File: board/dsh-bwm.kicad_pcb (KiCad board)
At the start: 2 copper layers, 137.4 x 88.5 mm, 67 parts, among them IC1 MAX485CSA+T, IC2 AT24C256C-SSHL-T, IC3 TPS5450DDA, J1 USB_A, J2 MPM-15-24, J3 Power, J4 LED, J5 SWD6p, J6 Connections, K1 T81N5D312, K2 T81N5D312, K3 T81N5D312, K4 T81N5D312, K5 T81N5D312, K6 T81N5D312, K7 T81N5D312, K8 T81N5D312, Q1 IRLB8721PBF, Q2 IRLB8721PBF, Q3 IRLB8721PBF, Q4 IRLB8721PBF, Q5 IRLB8721PBF, Q6 IRLB8721PBF, SW1 ModBus address selector, SW2 RESET, U1 RP2040_Stamp

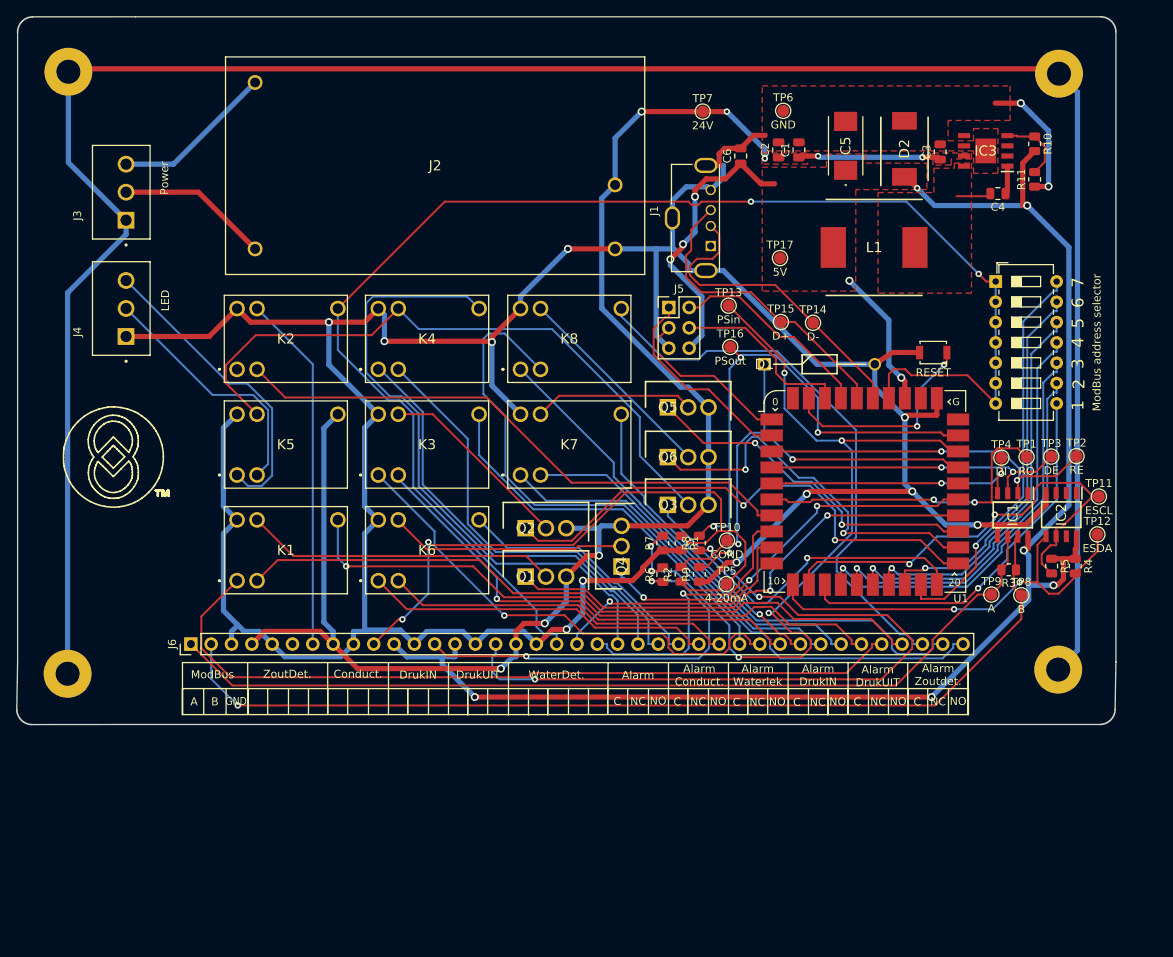
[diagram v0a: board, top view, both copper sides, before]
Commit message: pushpushpush
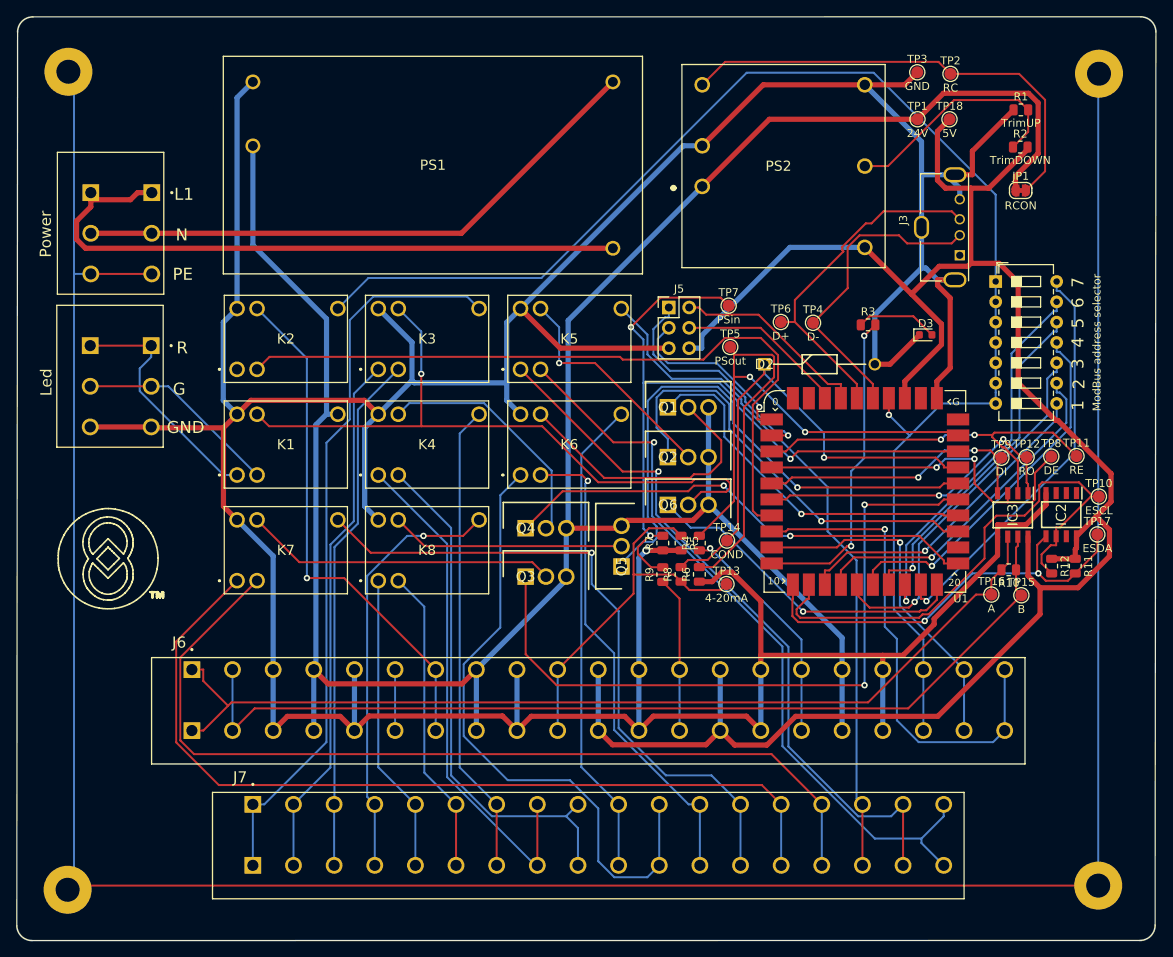
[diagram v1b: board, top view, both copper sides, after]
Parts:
- removed C1, C2: 4.7uF, Capacitor_SMD:C_0805_2012Metric
- removed C3, C4, C6: 0.01uF, Capacitor_SMD:C_0805_2012Metric
- removed C5: 330uF, SamacSys_Parts:POSCAP_D12_D15_D15E_D2E_D2_D3L_D4
- removed the D2 at (188.2, 69.8)
- removed the IC3 at (198.4, 70.1)
- removed J2: MPM-15-24, SamacSys_Parts:MPM1524
- removed L1: 15uH, SamacSys_Parts:INDPM120120X800N
- removed the R10 at (204.5, 69.2)
- removed the R11 at (204.5, 73.7)
- removed SW2: RESET, Button_Switch_SMD:SW_SPST_B3U-1000P
- removed the TP17 at (172.6, 83.5)
- added D3: LED_Small, LED_SMD:LED_0603_1608Metric, F.Cu at (190.8, 93.1)
- added J7: TBL004V-508-18BE-2GY, kicad_libs:CUI_TBL004V-508-18BE-2GY, F.Cu at (106.7, 151.8)
- added JP1: RCON, Jumper:SolderJumper-2_P1.3mm_Bridged_RoundedPad1.0x1.5mm, F.Cu at (202.7, 75.0)
- added PS1: MPM-15-24, SamacSys_Parts:MPM1524, F.Cu at (106.8, 69.5)
- added PS2: SKMW20F-05, SamacSys_Parts:SKMW20F05, F.Cu at (162.9, 74.5)
- added R1: TrimUP, Resistor_SMD:R_0805_2012Metric, F.Cu at (202.8, 65.0)
- added R2: TrimDOWN, Resistor_SMD:R_0805_2012Metric, F.Cu at (202.7, 69.6)
- added R3: 470, Resistor_SMD:R_0805_2012Metric, F.Cu at (183.7, 91.8)
- added TP18: 5V, TestPoint:TestPoint_Pad_D1.5mm, F.Cu at (193.8, 66.2)
- added TP2: RC, TestPoint:TestPoint_Pad_D1.5mm, F.Cu at (193.9, 60.5)
- J1: renamed from J3; footprint TBP03R2-350-03BE:CUI_TBP03R2-350-03BE -> kicad_libs:CUI_TBL004V-508-03BE-2GY
- J4: value LED -> Led; footprint TBP03R2-350-03BE:CUI_TBP03R2-350-03BE -> kicad_libs:CUI_TBL004V-508-03BE-2GY
- J6: value Connections -> TBL004V-508-21BE-2GY; footprint Connector_PinHeader_2.54mm:PinHeader_1x39_P2.54mm_Vertical -> kicad_libs:CUI_TBL004V-508-21BE-2GY
- moved J3 31.2 mm to (195.1, 83.2)
- moved H4 27.5 mm to (212.4, 161.9)
- moved H3 27.0 mm to (83.6, 162.5)
- moved TP1 26.9 mm to (189.8, 66.2)
- moved TP3 17.4 mm to (189.8, 60.3)
- moved H2 5.00 mm to (212.5, 60.5)
- moved J1 4.71 mm to (94.1, 75.3), turned to -90 degrees
- moved J4 3.34 mm to (94.0, 94.4), turned to -90 degrees
- moved J6 3.19 mm to (99.1, 134.9), turned to 0 degrees
- renumbered D1 to D2, H4 to H2, H2 to H4, IC1 to IC3, J1 to J3, K5 to K1, K4 to K3, K3 to K4, K8 to K5, K7 to K6, K1 to K7, K6 to K8, Q5 to Q1, Q6 to Q2, Q1 to Q3, Q2 to Q4, Q4 to Q5, Q3 to Q6, R3 to R10, R4 to R11, R5 to R12, R8 to R4, R1 to R5, R9 to R6, R2 to R8, R6 to R9, TP7 to TP1, TP11 to TP10, TP2 to TP11, TP1 to TP12, TP5 to TP13, TP10 to TP14, TP8 to TP15, TP9 to TP16, TP12 to TP17, TP6 to TP3, TP14 to TP4, TP16 to TP5, TP15 to TP6, TP13 to TP7, TP3 to TP8, TP4 to TP9
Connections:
- U1 pad 10: unconnected-(U1-Pad10) -> Net-(R3-Pad2)
- U1 pad 22: ALARMZOUT -> unconnected-(U1-Pad22)
- U1 pad 23: ALARMDRUKIN -> ALARMZOUT
- U1 pad 24: ALARMDRUKUIT -> ALARMDRUKIN
- U1 pad 25: ALARMCOND -> ALARMDRUKUIT
- U1 pad 26: unconnected-(U1-Pad26) -> ALARMCOND
- U1 pad 39: Net-(U1-Pad39) -> unconnected-(U1-Pad39)
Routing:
- net GND: track 409.6 -> 545.8 mm, vias 13 -> 1
- net 24V: track 201.6 -> 306.3 mm, vias 8 -> 0
- net PressureOUT: track 90.7 -> 29.0 mm, vias 3 -> 1
- net L1: track 20.4 -> 82.1 mm
- net Net-(H1-Pad1): track 281.9 -> 343.2 mm
- net Net-(PS2-Pad6): track 0.00 -> 58.3 mm
- net N: track 19.1 -> 73.1 mm
- net Net-(R3-Pad2): track 0.00 -> 39.8 mm, vias 0 -> 2
- net 4-20mA input: track 81.9 -> 47.1 mm, vias 2 -> 0
- net DrukInNC: track 46.6 -> 79.4 mm
- net PressureIN: track 50.4 -> 19.5 mm, vias 2 -> 0
- net Net-(PS2-Pad4): track 0.00 -> 29.8 mm
- net DrukUitNO: track 87.2 -> 115.1 mm
- net Net-(U1-Pad39): track 26.8 -> 0.00 mm, vias 2 -> 0
- net ALARMDRUKUIT: track 61.8 -> 88.2 mm
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- removed copper zone on F.Cu, net /Power/5Vunf
- removed copper zone on F.Cu, net 24V
- removed copper zone on F.Cu, net 5V
- removed copper zone on F.Cu, net GND
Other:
- board size 137.4 x 88.5 mm -> 142.4 x 115.5 mm
- board text added: "G"
- board text added: "L1"
- board text added: "N"
- board text added: "PE"
- board text added: "R"
- board text removed: "A"
- board text removed: "Alarm"
- board text removed: "Alarm Conduct."
- board text removed: "Alarm DrukIN"
- board text removed: "Alarm DrukUIT"
- board text removed: "Alarm Waterlek"
- board text removed: "Alarm Zoutdet."
- board text removed: "B"
- board text removed: "C"
- board text removed: "Conduct."
- board text removed: "DrukIN"
- board text removed: "DrukUIT"
- board text removed: "ModBus"
- board text removed: "NC"
- board text removed: "NO"
- board text removed: "WaterDet."
- board text removed: "ZoutDet."
